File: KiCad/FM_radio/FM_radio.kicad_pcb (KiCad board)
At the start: 2 copper layers, 33 x 48 mm, 77 parts, among them IC1 MCP73831T-2ACI_OT, IC2 SI4703-C19-GM, IC3 TPA741DR, IC4 TPA6111A2DR, J1 UJC-HP2-3-SMT-TR, J2 Conn_01x06_Pin, J3 SJ2-35853A-SMT-TR, U1 ATmega328P-A, Y1 ABS06N-32.768kHz-T

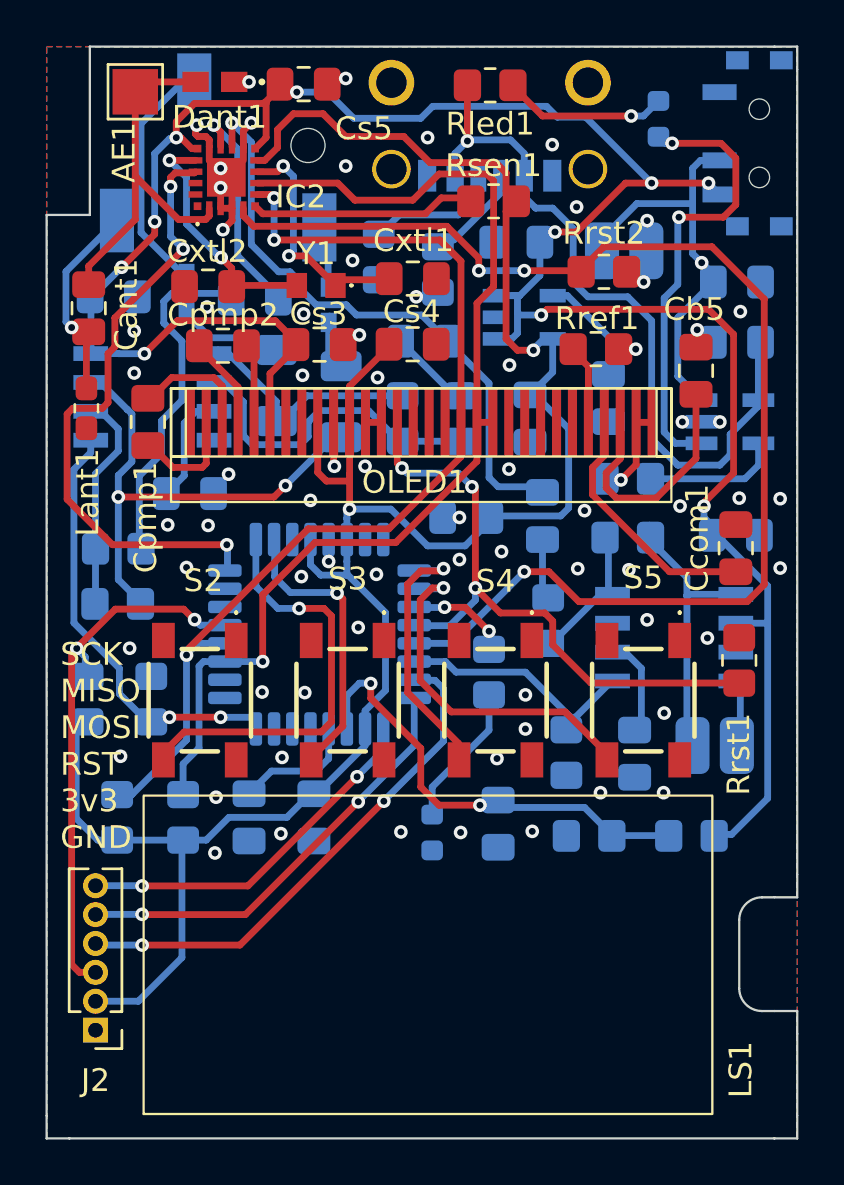
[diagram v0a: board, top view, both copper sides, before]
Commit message: Lant added
Last changes before JLC PCB
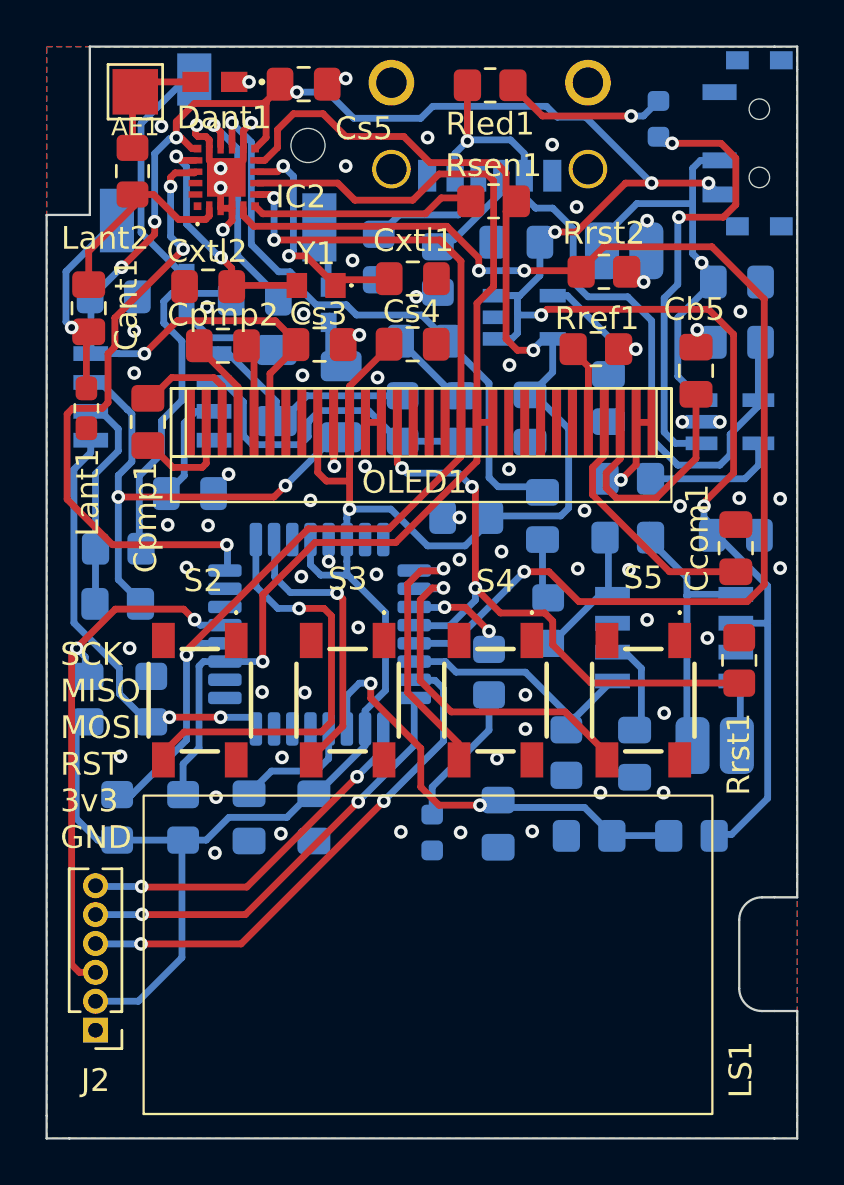
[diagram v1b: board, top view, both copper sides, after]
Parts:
- added Lant2: 350n, Inductor_SMD:L_0805_2012Metric_Pad1.15x1.40mm_HandSolder, F.Cu at (123.8, 75.5)
- turned Cc1 to 90 degrees
- turned Cc2 to 90 degrees
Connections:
- AE1 pad 1: /ANT -> Net-(AE1-A)
- Cc1 pad 1: Net-(Cc1-Pad1) -> Net-(IC4-VO1)
- Cc1 pad 2: Net-(IC4-VO1) -> Net-(Cc1-Pad2)
- Cc2 pad 1: Net-(Cc2-Pad1) -> Net-(IC4-VO2)
- Cc2 pad 2: Net-(IC4-VO2) -> Net-(Cc2-Pad2)
- Dant1 pad 2: /ANT -> Net-(AE1-A)
- FB1 pad 1: Net-(Cc1-Pad1) -> Net-(Cc1-Pad2)
- FB2 pad 2: Net-(Cc2-Pad1) -> Net-(Cc2-Pad2)
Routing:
- net /ANT: track 16.7 -> 9.06 mm
- net Net-(AE1-A): track 0.00 -> 5.58 mm
- net Net-(Cc1-Pad2): track 0.00 -> 4.83 mm
- net Net-(Cc1-Pad1): track 4.83 -> 0.00 mm
- net Net-(Cc2-Pad2): track 0.00 -> 2.46 mm
- net Net-(Cc2-Pad1): track 2.46 -> 0.00 mm
- net GND: vias 70 -> 71
